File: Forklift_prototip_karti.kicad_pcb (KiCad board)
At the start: 2 copper layers, 25 parts, among them J10 Mini360, J11 Barrel_Jack_Switch, J6 Conn_01x22_Pin, J7 Conn_01x22_Pin, U1 ESP32-S3-DEVKITC-1-N8R2, U2 PCF8563T, Y1 32.768 KHz

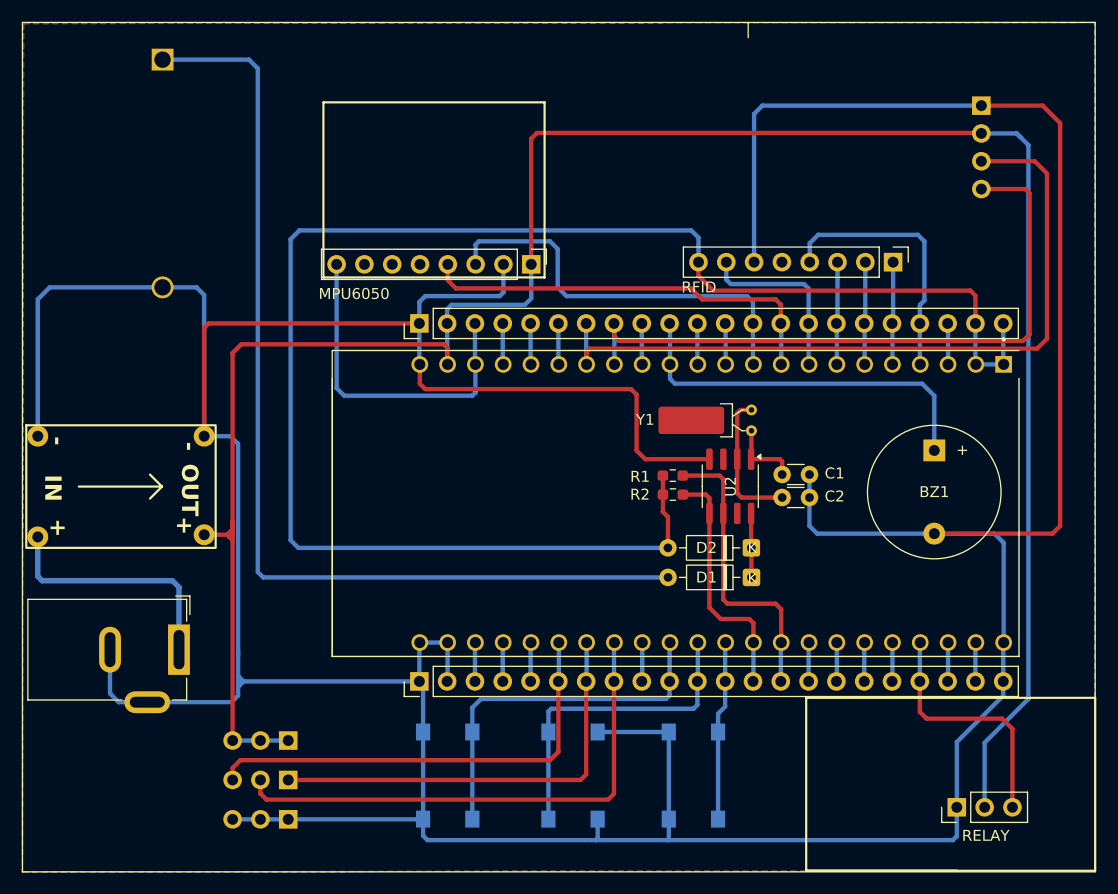
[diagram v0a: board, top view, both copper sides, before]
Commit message: Add files via upload
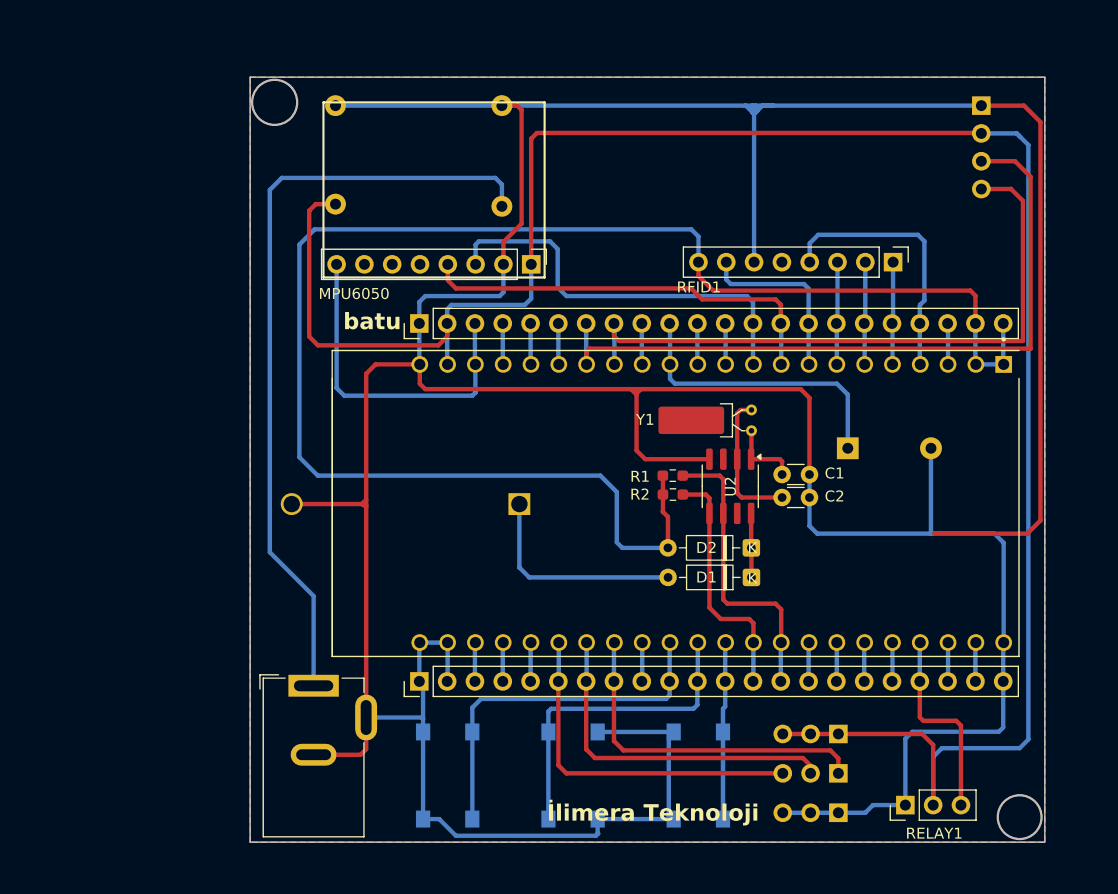
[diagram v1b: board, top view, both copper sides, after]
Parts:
- BZ1, J10: moved to B.Cu
- moved BT1 52.1 mm to (142.2, 79.1), turned to 180 degrees
- moved GND1 50.3 mm to (171.3, 107.3)
- moved SKB 50.3 mm to (171.3, 103.7)
- moved VCC1 50.3 mm to (171.3, 100.1)
- moved J10 40.8 mm to (133.1, 47.2), turned to 180 degrees
- moved J11 12.7 mm to (123.4, 95.7), turned to 0 degrees
- moved BZ1 7.90 mm to (172.2, 74.0), turned to 0 degrees
- moved RELAY1 4.70 mm to (177.5, 106.6)
- moved B37 0.45 mm to (158.6, 103.9)
- renumbered GND to GND1, LCD to LCD1, RELAY to RELAY1, RFID to RFID1, VCC to VCC1
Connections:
- SKB pad 1: /IO48 -> /IO45
- SKB pad 2: /IO45 -> /IO48
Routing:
- net Net-(BT1-+): track 92.7 -> 19.8 mm
- net /Vin: track 22.6 -> 70.9 mm
- net GND: track 434.8 -> 415.9 mm
- net /IO45: track 47.8 -> 31.5 mm
- net /5V: track 203.2 -> 190.7 mm
- net /IO47: track 41.5 -> 32.0 mm
- net /IO3: track 34.9 -> 26.8 mm
- net /IO48: track 39.5 -> 31.6 mm
- net /IO1: track 22.6 -> 18.2 mm
- net /3V3: track 149.4 -> 145.9 mm
- net /IO10: track 69.1 -> 66.4 mm
- net /IO9: track 60.8 -> 59.5 mm
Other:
- board outline added: 72.6 x 69.9 mm
- board text added: "batu"
- board text added: "İlimera Teknoloji"
